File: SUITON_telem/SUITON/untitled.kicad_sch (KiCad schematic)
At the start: 18 parts, among them U2 ISM330DHCXTR, U3 MMC5983MA, U4 SAM-M10Q-00B, U5 BMP581, U8 LSM6DSV320XTR

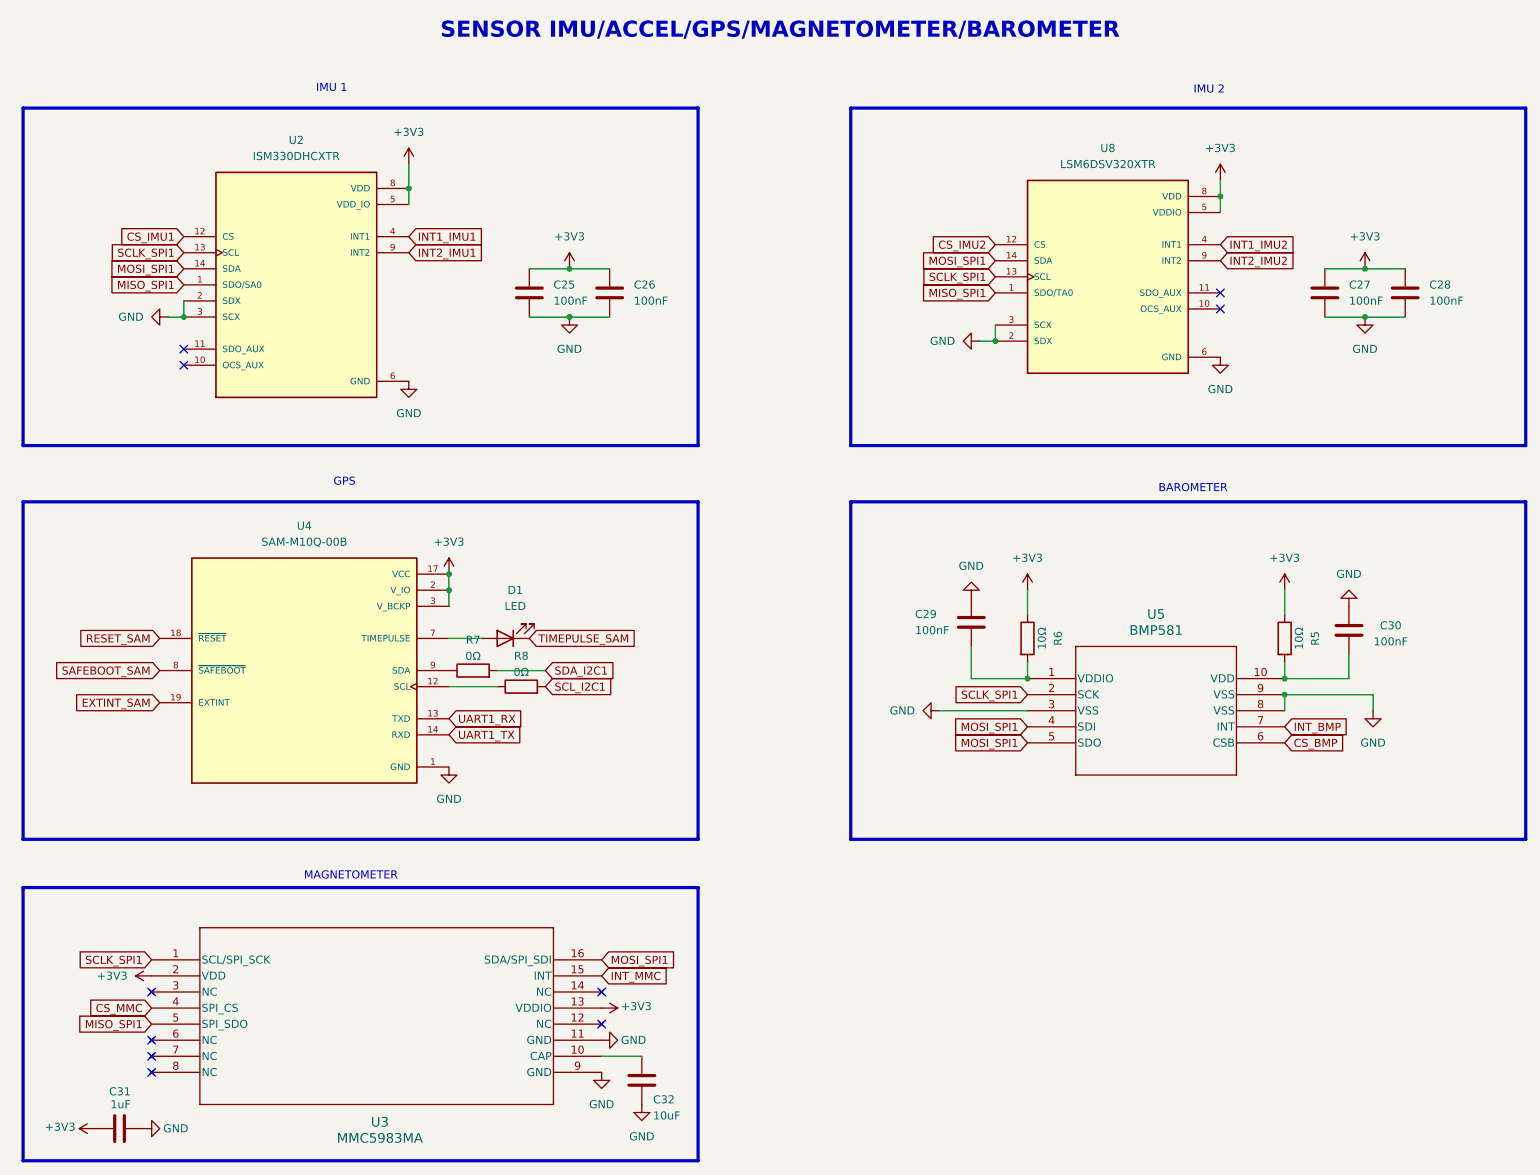
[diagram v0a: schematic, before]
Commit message: power management
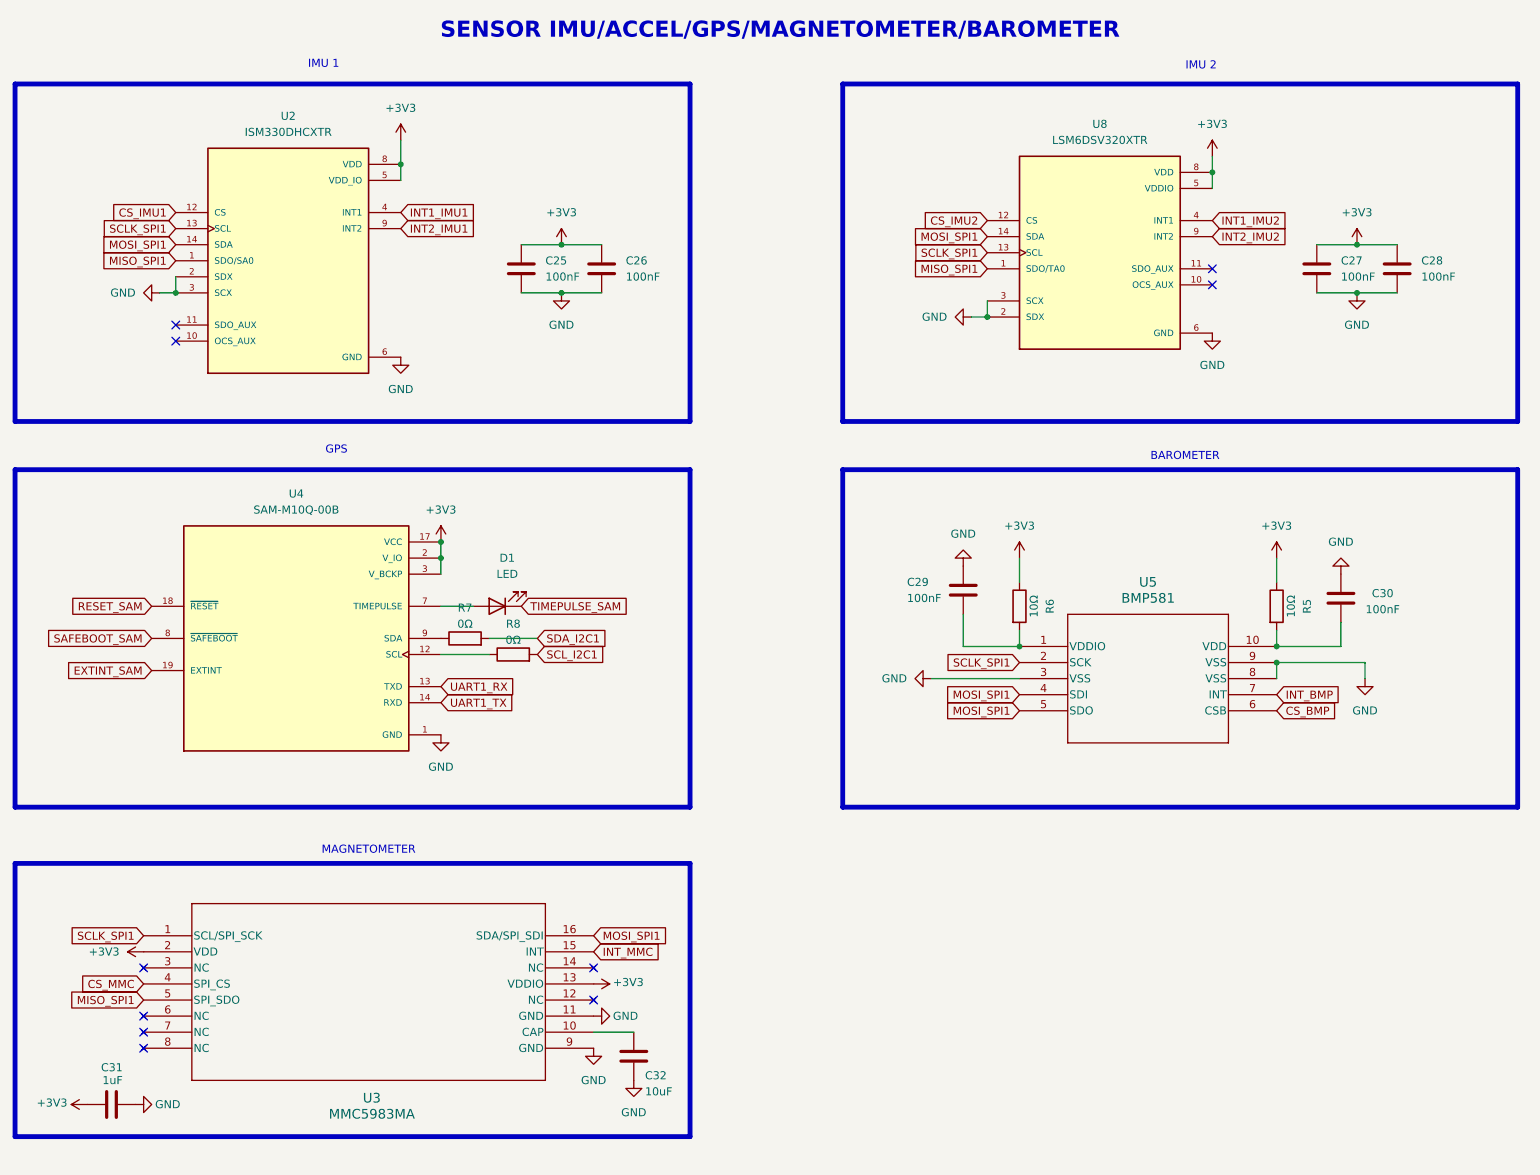
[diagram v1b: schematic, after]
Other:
- company: (none) -> S.T.A.R.
- title: (none) -> SUITON PRO
- moved on the sheet: C25, C26, C27, C28, C29, C30, C31, C32, D1, R5, R6, R7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
